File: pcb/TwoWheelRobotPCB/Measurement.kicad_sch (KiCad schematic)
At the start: 8 parts, among them U5 TXB0104D, U6 MCP3004, U7 ACS712_M1, U8 ACS712_M2

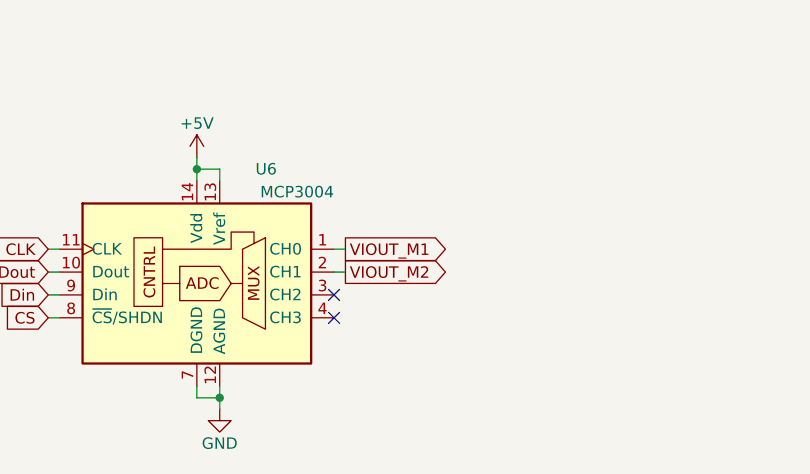
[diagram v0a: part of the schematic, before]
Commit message: update pcb
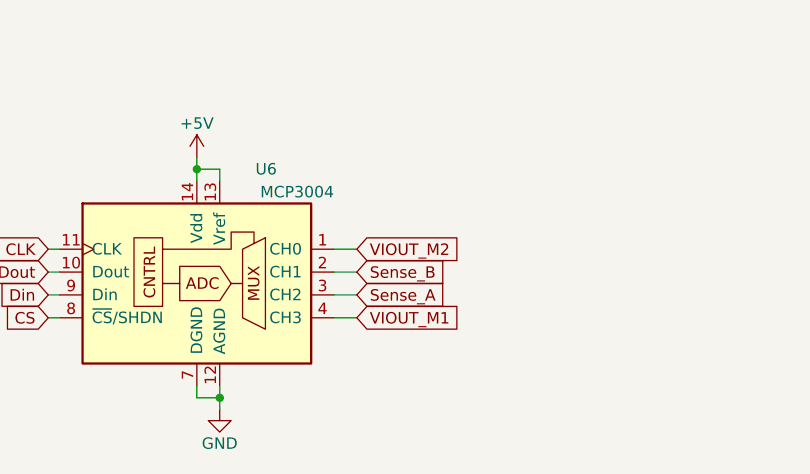
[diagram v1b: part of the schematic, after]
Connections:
- net VIOUT_M1: now also U6.4 (CH3); no longer U6.1 (CH0)
- net VIOUT_M2: now also U6.1 (CH0); no longer U6.2 (CH1)
- net Sense_A: now reaches U6.3 (CH2)
- new net Sense_B: U6.2 (CH1)
- no-connect marks 2 -> 0
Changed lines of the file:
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@@
   (junction (at 208.28 74.93) (diameter 0) (color 0 0 0 0)
   )
-  (no_connect (at 133.35 121.92))
-  (no_connect (at 133.35 119.38))
   (wire (pts (xy 191.77 101.6) (xy 191.77 100.33))
     (stroke (width 0) (type default) (color 0 0 0 0))
@@
     (stroke (width 0) (type default) (color 0 0 0 0))
   )
-  (wire (pts (xy 134.62 116.84) (xy 133.35 116.84))
-    (stroke (width 0) (type default) (color 0 0 0 0))
-  )
   (wire (pts (xy 219.71 62.23) (xy 218.44 62.23))
     (stroke (width 0) (type default) (color 0 0 0 0))
   )
+  (wire (pts (xy 135.89 119.38) (xy 133.35 119.38))
+    (stroke (width 0) (type default) (color 0 0 0 0))
+  )
   (wire (pts (xy 115.57 39.37) (xy 115.57 41.91))
     (stroke (width 0) (type default) (color 0 0 0 0))
@@
     (stroke (width 0) (type default) (color 0 0 0 0))
   )
+  (wire (pts (xy 135.89 121.92) (xy 133.35 121.92))
+    (stroke (width 0) (type default) (color 0 0 0 0))
+  )
   (wire (pts (xy 208.28 39.37) (xy 208.28 44.45))
     (stroke (width 0) (type default) (color 0 0 0 0))
@@
     (stroke (width 0) (type default) (color 0 0 0 0))
   )
+  (wire (pts (xy 135.89 116.84) (xy 133.35 116.84))
+    (stroke (width 0) (type default) (color 0 0 0 0))
+  )
   (wire (pts (xy 110.49 40.64) (xy 110.49 41.91))
     (stroke (width 0) (type default) (color 0 0 0 0))
@@
     (stroke (width 0) (type default) (color 0 0 0 0))
   )
+  (wire (pts (xy 135.89 114.3) (xy 133.35 114.3))
+    (stroke (width 0) (type default) (color 0 0 0 0))
+  )
   (wire (pts (xy 124.46 52.07) (xy 123.19 52.07))
     (stroke (width 0) (type default) (color 0 0 0 0))
@@
     (stroke (width 0) (type default) (color 0 0 0 0))
   )
-  (wire (pts (xy 134.62 114.3) (xy 133.35 114.3))
-    (stroke (width 0) (type default) (color 0 0 0 0))
-  )
   (wire (pts (xy 102.87 119.38) (xy 101.6 119.38))
     (stroke (width 0) (type default) (color 0 0 0 0))
@@
     )
   )
+  (global_label "Sense_A" (shape input) (at 135.89 119.38 0) (fields_autoplaced)
+    (effects (font (size 1.27 1.27)) (justify left))
+    (property "Intersheet References" "${INTERSHEET_REFS}" (id 0) (at 145.9231 119.3006 0)
+      (effects (font (size 1.27 1.27)) (justify left) hide)
+    )
+  )
   (global_label "OUT1" (shape input) (at 196.85 54.61 180) (fields_autoplaced)
     (effects (font (size 1.27 1.27)) (justify right))
@@
     )
   )
+  (global_label "Sense_B" (shape input) (at 135.89 116.84 0) (fields_autoplaced)
+    (effects (font (size 1.27 1.27)) (justify left))
+    (property "Intersheet References" "${INTERSHEET_REFS}" (id 0) (at 146.1045 116.7606 0)
+      (effects (font (size 1.27 1.27)) (justify left) hide)
+    )
+  )
   (global_label "Din" (shape input) (at 101.6 119.38 180) (fields_autoplaced)
     (effects (font (size 1.27 1.27)) (justify right))
@@
     )
   )
-  (global_label "VIOUT_M2" (shape output) (at 134.62 116.84 0) (fields_autoplaced)
-    (effects (font (size 1.27 1.27)) (justify left))
-    (property "Intersheet References" "${INTERSHEET_REFS}" (id 0) (at 145.9836 116.9194 0)
+  (global_label "VIOUT_M2" (shape input) (at 135.89 114.3 0) (fields_autoplaced)
+    (effects (font (size 1.27 1.27)) (justify left))
+    (property "Intersheet References" "${INTERSHEET_REFS}" (id 0) (at 147.2536 114.2206 0)
       (effects (font (size 1.27 1.27)) (justify left) hide)
     )
@@
     )
   )
-  (global_label "VIOUT_M1" (shape output) (at 134.62 114.3 0) (fields_autoplaced)
-    (effects (font (size 1.27 1.27)) (justify left))
-    (property "Intersheet References" "${INTERSHEET_REFS}" (id 0) (at 145.9836 114.3794 0)
-      (effects (font (size 1.27 1.27)) (justify left) hide)
-    )
+  (global_label "VIOUT_M1" (shape input) (at 135.89 121.92 0) (fields_autoplaced)
+    (effects (font (size 1.27 1.27)) (justify left))
+    (property "Intersheet References" "${INTERSHEET_REFS}" (id 0) (at 147.2536 121.8406 0)
+      (effects (font (size 1.27 1.27)) (justify left) hide)
+    )
